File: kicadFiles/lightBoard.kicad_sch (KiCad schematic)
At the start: 24 parts, among them J1 Screw_Terminal_01x02, J2 Screw_Terminal_01x02, J3 Screw_Terminal_01x02, J4 Screw_Terminal_01x02, J5 Screw_Terminal_01x02, J6 Screw_Terminal_01x02, J7 Screw_Terminal_01x02, Q1 2N7002, Q2 2N7002, Q4 2N7002, Q5 2N7002, Q6 2N7002, U1 ATtiny85-20P

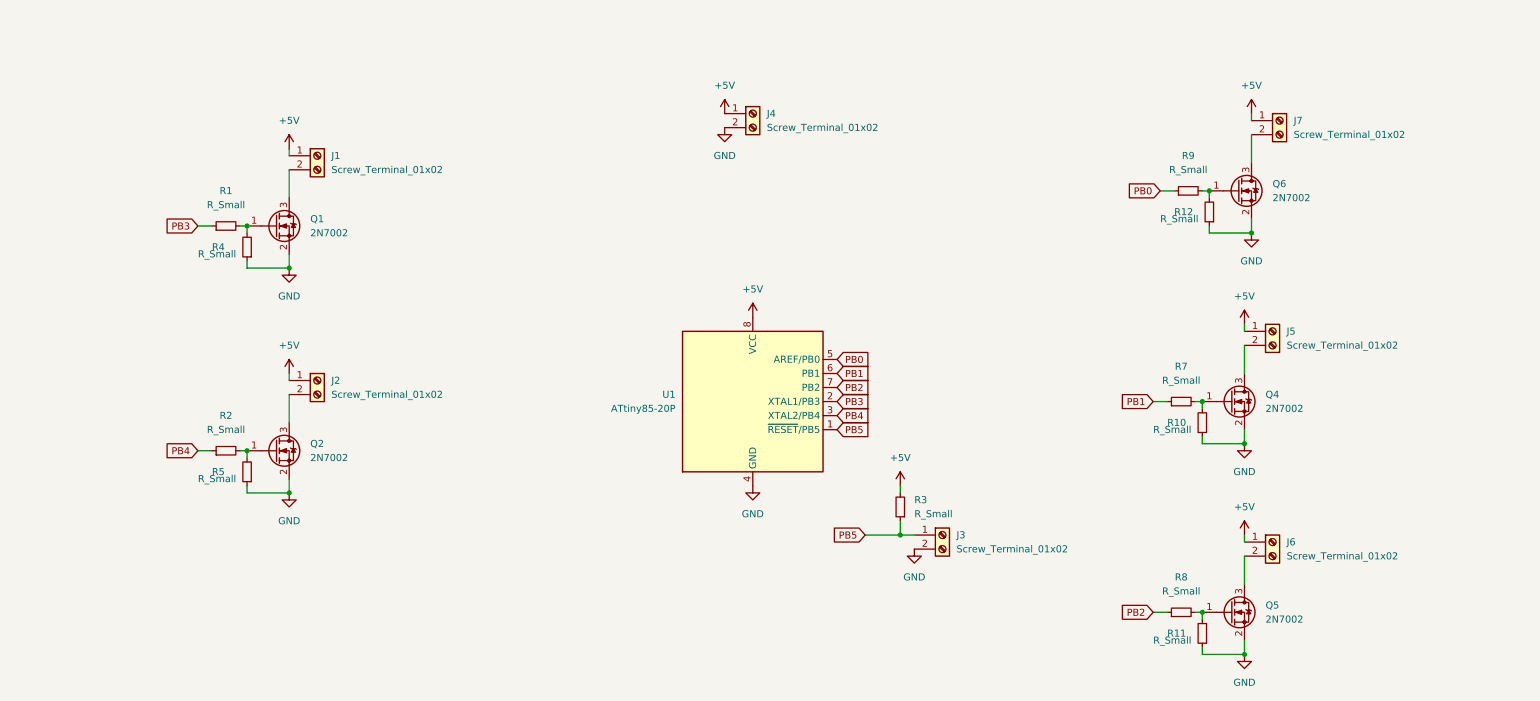
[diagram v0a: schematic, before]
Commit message: Added pdf
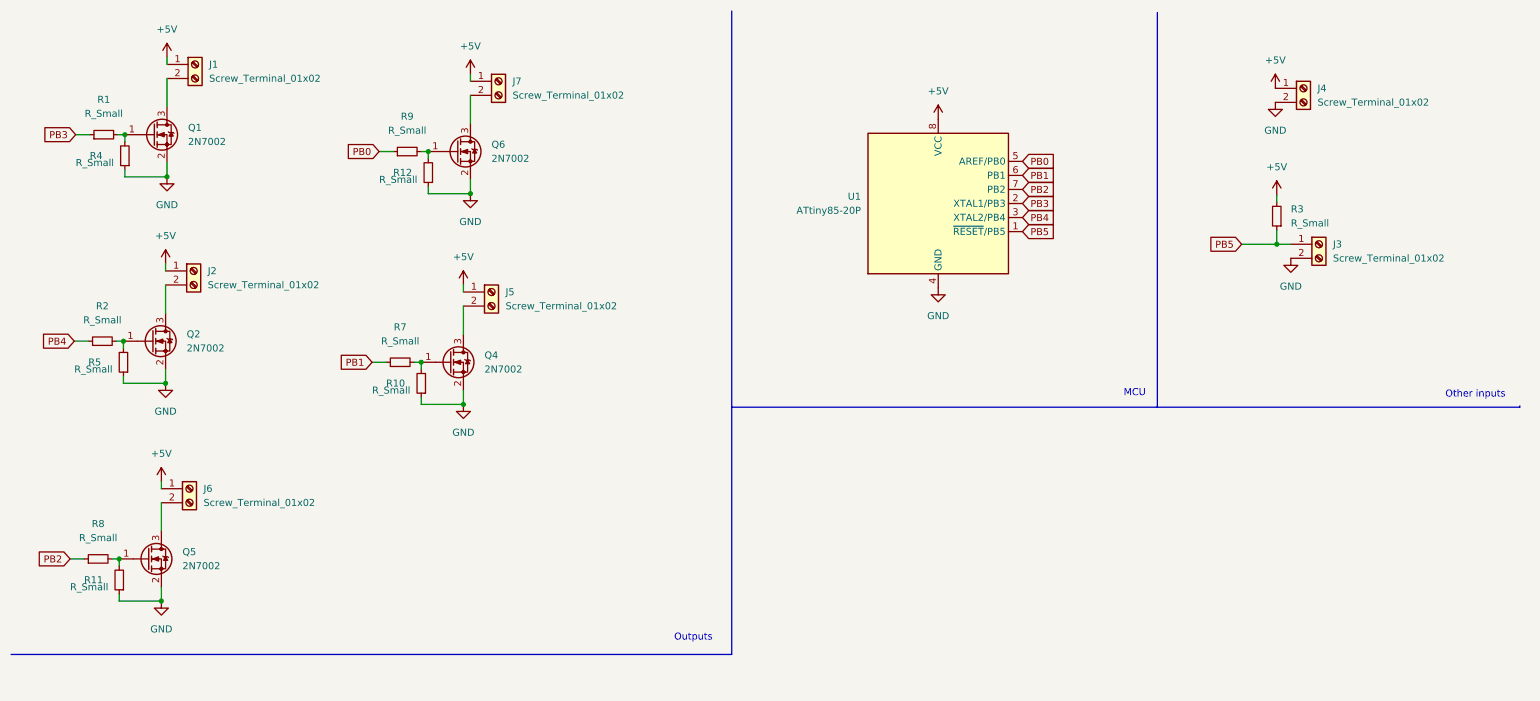
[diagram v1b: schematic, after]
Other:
- note added: "MCU"
- note added: "Other inputs"
- note added: "Outputs"
- moved on the sheet: J1, J2, J3, J4, J5, J6, J7, Q1, Q2, Q4, Q5, Q6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
